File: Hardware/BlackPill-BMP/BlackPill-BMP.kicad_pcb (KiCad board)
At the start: 2 copper layers, 72.5 x 59.7 mm, 41 parts, among them J1 JTAG, J10 Conn_01x12_Male, J2 VCC, J3 GND, J4 SWO, J5 GDB_COMM, J6 TVCC, J7 LogicAna, J8 Conn_01x06_Male, J9 Conn_01x05_Male, U1 BlueAndBlackPill, U2 AD8531ARTZ, U3 74LVC2T45DC, U4 74LS126, U5 74LS126, U6 SRV05-4, U7 SRV05-4

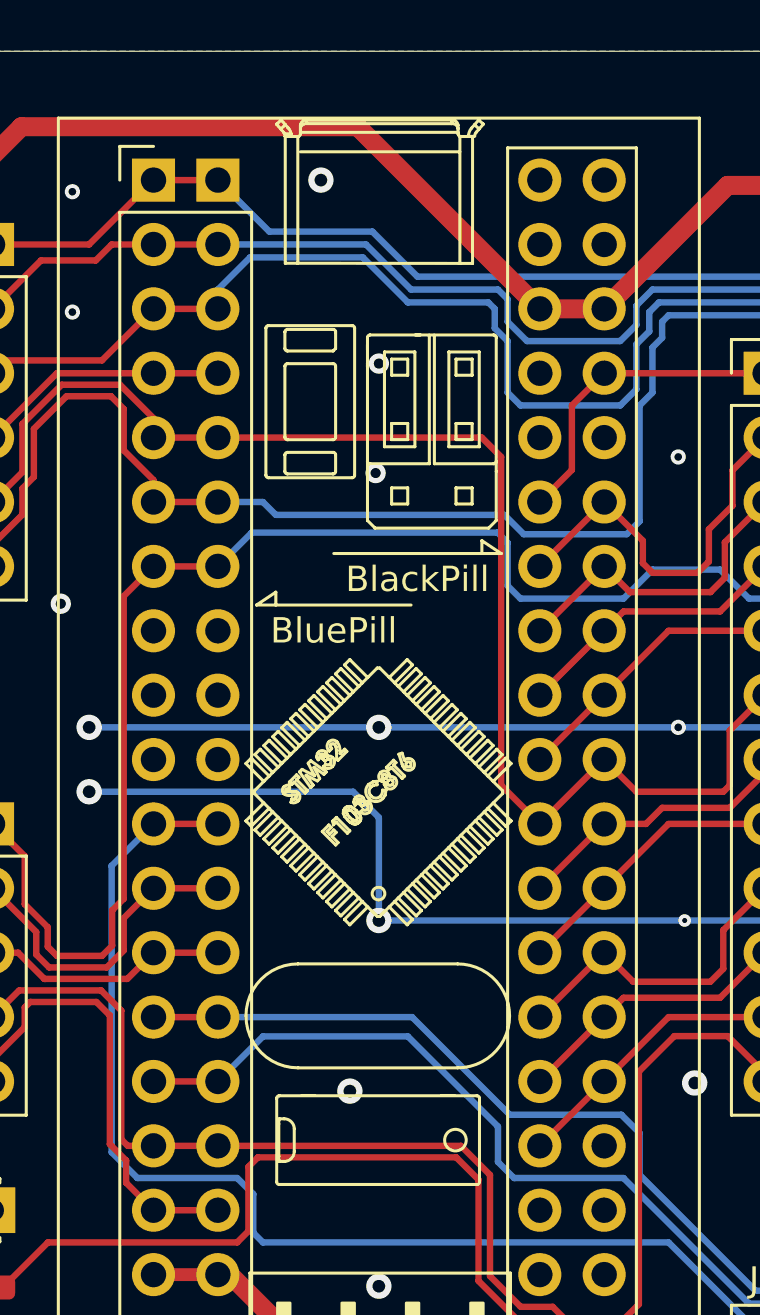
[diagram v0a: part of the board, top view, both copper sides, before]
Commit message: - Components review
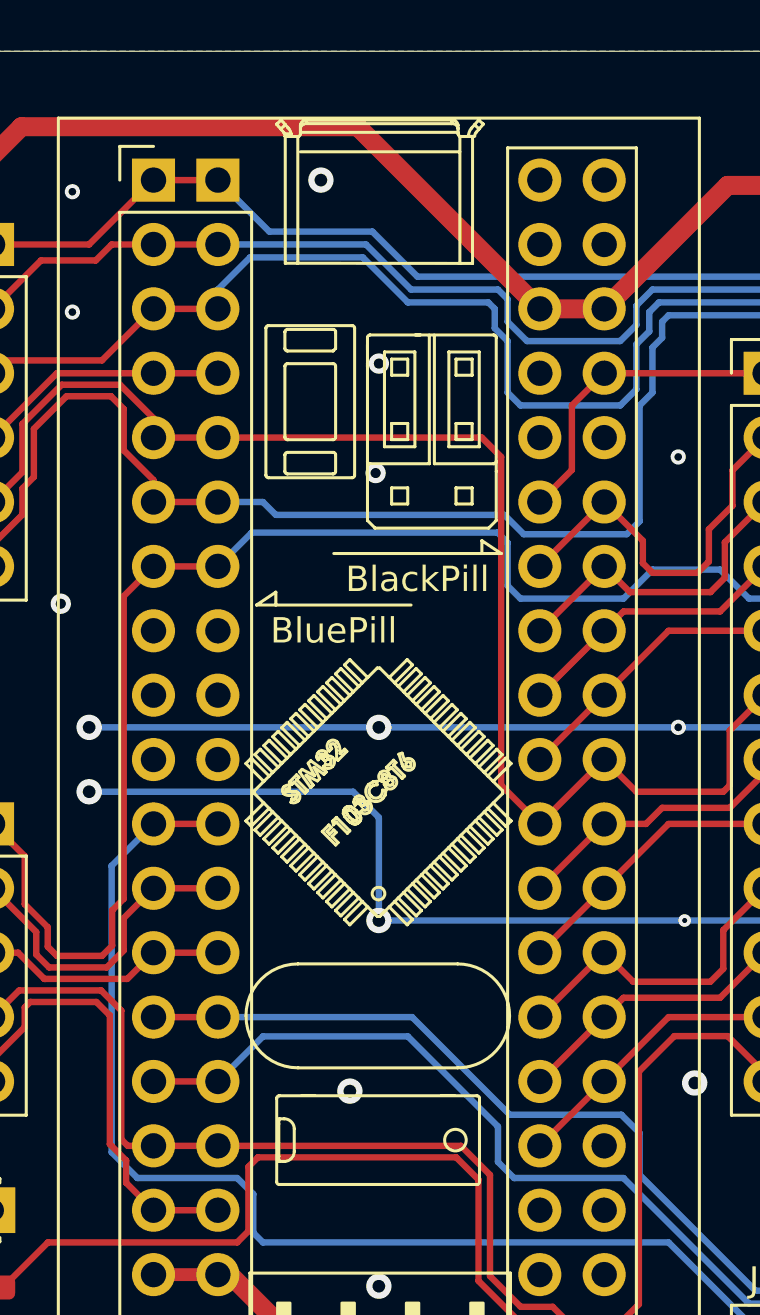
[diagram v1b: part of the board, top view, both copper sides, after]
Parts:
- RN3, RN5: value 47 -> 100
